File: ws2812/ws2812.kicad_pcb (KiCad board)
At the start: 2 copper layers, 76.2 x 50.8 mm, 8 parts, among them J1 STM32WORLD_BASE, J2 STM32WORLD_CONNECTOR_1, J3 STM32WORLD_CONNECTOR_2, U1 WS2812E, U2 WS2812E, U3 WS2812E, U4 WS2812E, U5 WS2812E

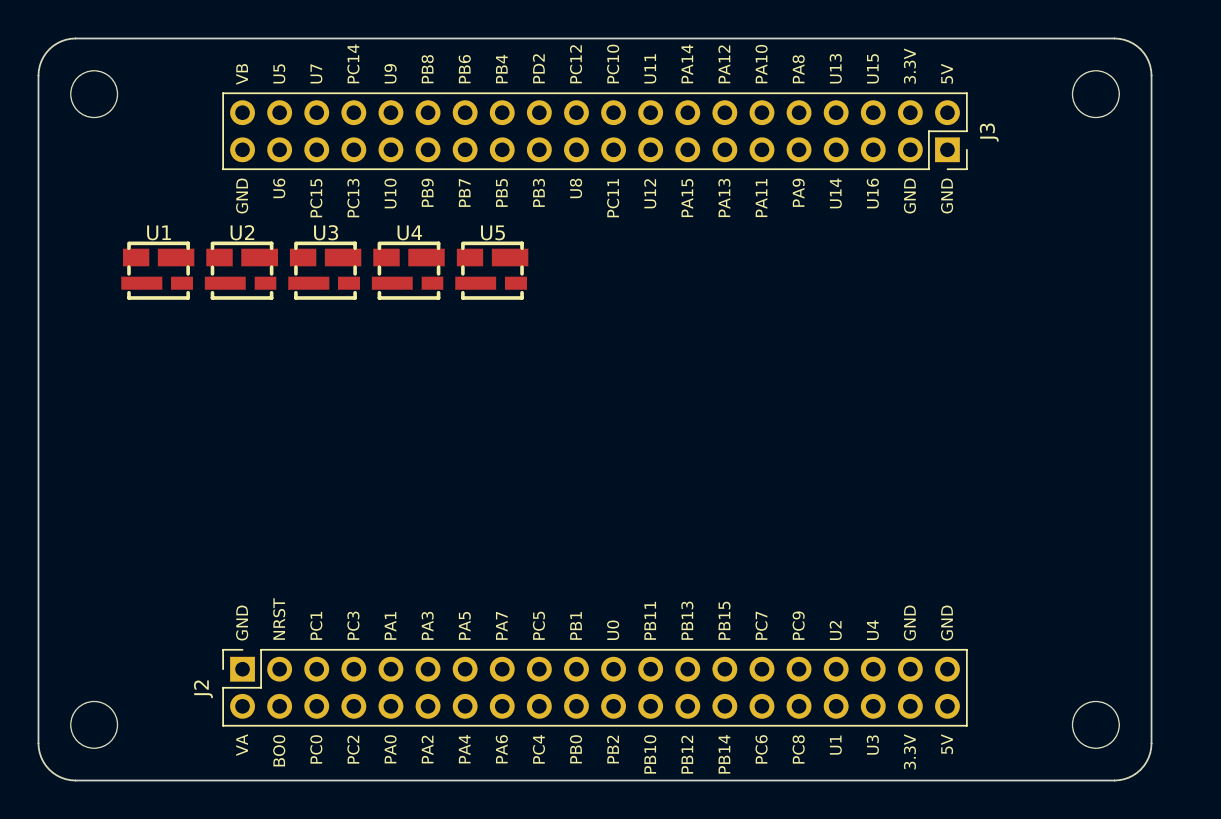
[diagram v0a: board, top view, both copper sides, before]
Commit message: Hmmmm
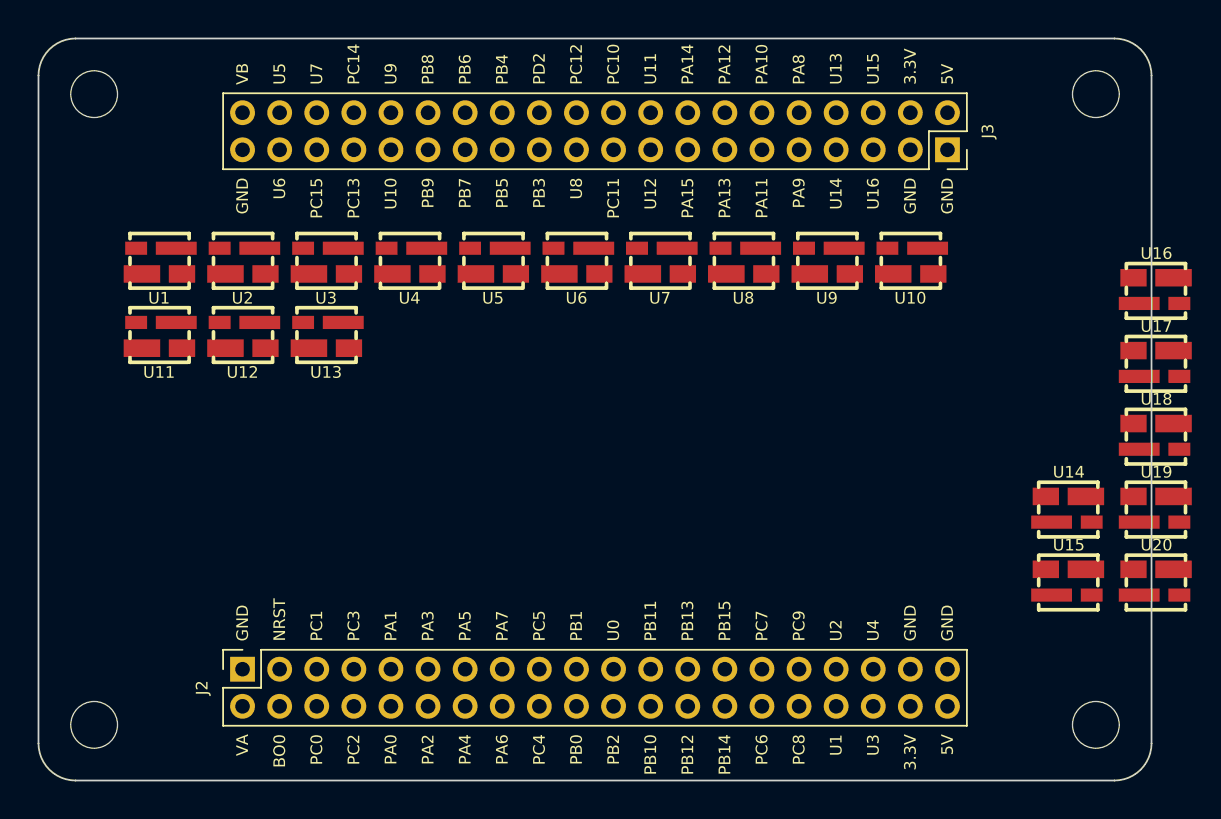
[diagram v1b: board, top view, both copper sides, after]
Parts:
- added U10: WS2812E, stm32world:LED-SMD_4P-L3.7-W3.5-P1.75-BR-SK6812MINI, F.Cu at (167.6, 85.1)
- added U11: WS2812E, stm32world:LED-SMD_4P-L3.7-W3.5-P1.75-BR-SK6812MINI, F.Cu at (116.2, 90.2)
- added U12: WS2812E, stm32world:LED-SMD_4P-L3.7-W3.5-P1.75-BR-SK6812MINI, F.Cu at (121.9, 90.2)
- added U13: WS2812E, stm32world:LED-SMD_4P-L3.7-W3.5-P1.75-BR-SK6812MINI, F.Cu at (127.6, 90.2)
- added U14: WS2812E, stm32world:LED-SMD_4P-L3.7-W3.5-P1.75-BR-SK6812MINI, F.Cu at (178.5, 102.1)
- added U15: WS2812E, stm32world:LED-SMD_4P-L3.7-W3.5-P1.75-BR-SK6812MINI, F.Cu at (178.5, 107.1)
- added U16: WS2812E, stm32world:LED-SMD_4P-L3.7-W3.5-P1.75-BR-SK6812MINI, F.Cu at (184.5, 87.1)
- added U17: WS2812E, stm32world:LED-SMD_4P-L3.7-W3.5-P1.75-BR-SK6812MINI, F.Cu at (184.5, 92.1)
- added U18: WS2812E, stm32world:LED-SMD_4P-L3.7-W3.5-P1.75-BR-SK6812MINI, F.Cu at (184.5, 97.1)
- added U19: WS2812E, stm32world:LED-SMD_4P-L3.7-W3.5-P1.75-BR-SK6812MINI, F.Cu at (184.5, 102.1)
- added U20: WS2812E, stm32world:LED-SMD_4P-L3.7-W3.5-P1.75-BR-SK6812MINI, F.Cu at (184.5, 107.1)
- added U6: WS2812E, stm32world:LED-SMD_4P-L3.7-W3.5-P1.75-BR-SK6812MINI, F.Cu at (144.8, 85.1)
- added U7: WS2812E, stm32world:LED-SMD_4P-L3.7-W3.5-P1.75-BR-SK6812MINI, F.Cu at (150.5, 85.1)
- added U8: WS2812E, stm32world:LED-SMD_4P-L3.7-W3.5-P1.75-BR-SK6812MINI, F.Cu at (156.2, 85.1)
- added U9: WS2812E, stm32world:LED-SMD_4P-L3.7-W3.5-P1.75-BR-SK6812MINI, F.Cu at (161.9, 85.1)
- J1: value STM32WORLD_BASE -> STM32WORLD_BOARD
- moved U1 0.63 mm to (116.2, 85.1), turned to 180 degrees
- moved U2 0.63 mm to (121.9, 85.1), turned to 180 degrees
- moved U3 0.63 mm to (127.6, 85.1), turned to 180 degrees
- moved U4 0.63 mm to (133.3, 85.1), turned to 180 degrees
- moved U5 0.63 mm to (139.1, 85.1), turned to 180 degrees
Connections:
- U1 pad 2: unconnected-(U1-VDD-Pad2) -> VCC
- U1 pad 3: unconnected-(U1-DO-Pad3) -> Net-(U1-DO)
- U1 pad 4: unconnected-(U1-GND-Pad4) -> GND
- U2 pad 1: unconnected-(U2-DI-Pad1) -> Net-(U1-DO)
- U2 pad 2: unconnected-(U2-VDD-Pad2) -> VCC
- U2 pad 3: unconnected-(U2-DO-Pad3) -> Net-(U2-DO)
- U2 pad 4: unconnected-(U2-GND-Pad4) -> GND
- U3 pad 1: unconnected-(U3-DI-Pad1) -> Net-(U2-DO)
- U3 pad 2: unconnected-(U3-VDD-Pad2) -> VCC
- U3 pad 3: unconnected-(U3-DO-Pad3) -> Net-(U3-DO)
- U3 pad 4: unconnected-(U3-GND-Pad4) -> GND
- U4 pad 1: unconnected-(U4-DI-Pad1) -> Net-(U3-DO)
- U4 pad 2: unconnected-(U4-VDD-Pad2) -> VCC
- U4 pad 3: unconnected-(U4-DO-Pad3) -> Net-(U4-DO)
- U4 pad 4: unconnected-(U4-GND-Pad4) -> GND
- U5 pad 1: unconnected-(U5-DI-Pad1) -> Net-(U4-DO)
- U5 pad 2: unconnected-(U5-VDD-Pad2) -> VCC
- U5 pad 3: unconnected-(U5-DO-Pad3) -> Net-(U5-DO)
- U5 pad 4: unconnected-(U5-GND-Pad4) -> GND

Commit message: More
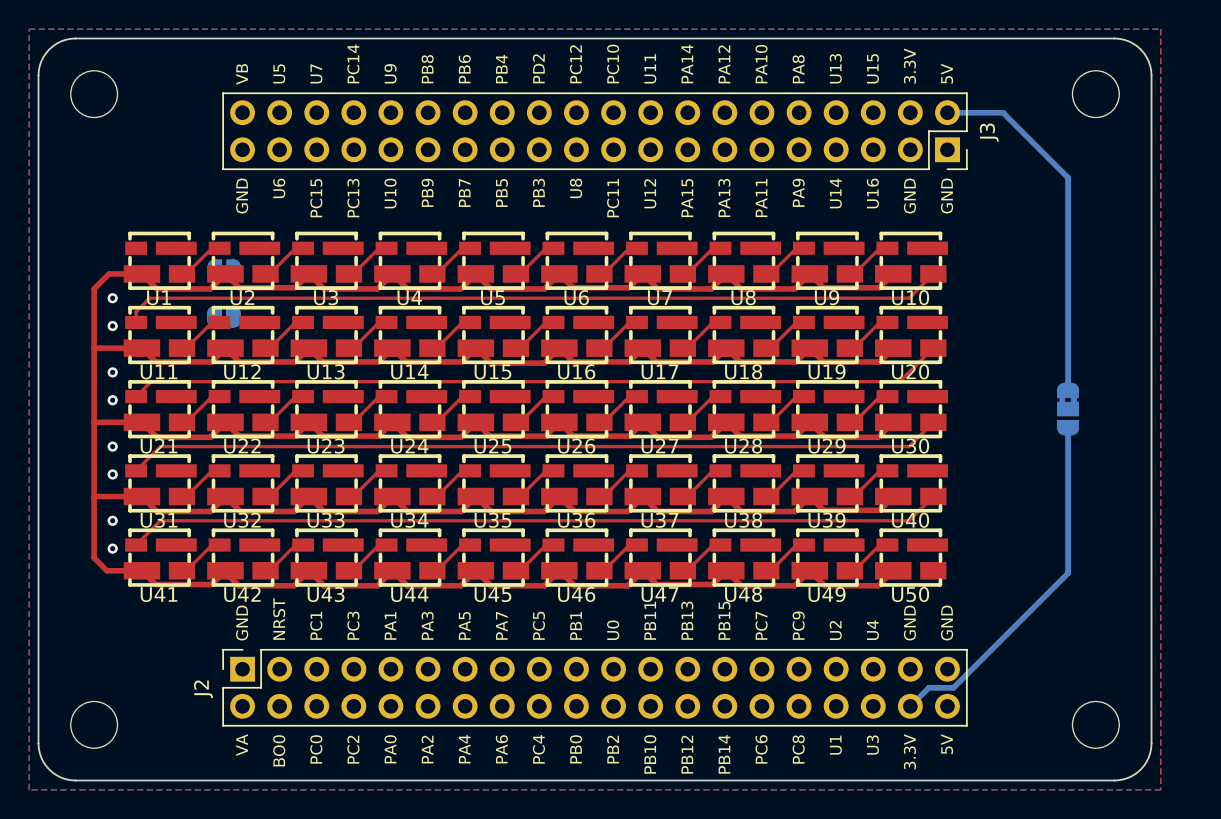
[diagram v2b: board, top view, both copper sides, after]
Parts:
- added JP1: ~, Jumper:SolderJumper-3_P1.3mm_Bridged2Bar12_RoundedPad1.0x1.5mm, B.Cu at (178.4, 95.2)
- added JP2: ~, Jumper:SolderJumper-2_P1.3mm_Open_RoundedPad1.0x1.5mm, B.Cu at (120.7, 85.7)
- added JP3: ~, Jumper:SolderJumper-2_P1.3mm_Open_RoundedPad1.0x1.5mm, B.Cu at (120.7, 88.9)
- added U21: WS2812E, stm32world:LED-SMD_4P-L3.7-W3.5-P1.75-BR-SK6812MINI, F.Cu at (116.2, 95.2)
- added U22: WS2812E, stm32world:LED-SMD_4P-L3.7-W3.5-P1.75-BR-SK6812MINI, F.Cu at (121.9, 95.2)
- added U23: WS2812E, stm32world:LED-SMD_4P-L3.7-W3.5-P1.75-BR-SK6812MINI, F.Cu at (127.6, 95.2)
- added U24: WS2812E, stm32world:LED-SMD_4P-L3.7-W3.5-P1.75-BR-SK6812MINI, F.Cu at (133.3, 95.2)
- added U25: WS2812E, stm32world:LED-SMD_4P-L3.7-W3.5-P1.75-BR-SK6812MINI, F.Cu at (139.1, 95.2)
- added U26: WS2812E, stm32world:LED-SMD_4P-L3.7-W3.5-P1.75-BR-SK6812MINI, F.Cu at (144.8, 95.2)
- added U27: WS2812E, stm32world:LED-SMD_4P-L3.7-W3.5-P1.75-BR-SK6812MINI, F.Cu at (150.5, 95.2)
- added U28: WS2812E, stm32world:LED-SMD_4P-L3.7-W3.5-P1.75-BR-SK6812MINI, F.Cu at (156.2, 95.2)
- added U29: WS2812E, stm32world:LED-SMD_4P-L3.7-W3.5-P1.75-BR-SK6812MINI, F.Cu at (161.9, 95.2)
- added U30: WS2812E, stm32world:LED-SMD_4P-L3.7-W3.5-P1.75-BR-SK6812MINI, F.Cu at (167.6, 95.2)
- added U31: WS2812E, stm32world:LED-SMD_4P-L3.7-W3.5-P1.75-BR-SK6812MINI, F.Cu at (116.2, 100.3)
- added U32: WS2812E, stm32world:LED-SMD_4P-L3.7-W3.5-P1.75-BR-SK6812MINI, F.Cu at (121.9, 100.3)
- added U33: WS2812E, stm32world:LED-SMD_4P-L3.7-W3.5-P1.75-BR-SK6812MINI, F.Cu at (127.6, 100.3)
- added U34: WS2812E, stm32world:LED-SMD_4P-L3.7-W3.5-P1.75-BR-SK6812MINI, F.Cu at (133.3, 100.3)
- added U35: WS2812E, stm32world:LED-SMD_4P-L3.7-W3.5-P1.75-BR-SK6812MINI, F.Cu at (139.1, 100.3)
- added U36: WS2812E, stm32world:LED-SMD_4P-L3.7-W3.5-P1.75-BR-SK6812MINI, F.Cu at (144.8, 100.3)
- added U37: WS2812E, stm32world:LED-SMD_4P-L3.7-W3.5-P1.75-BR-SK6812MINI, F.Cu at (150.5, 100.3)
- added U38: WS2812E, stm32world:LED-SMD_4P-L3.7-W3.5-P1.75-BR-SK6812MINI, F.Cu at (156.2, 100.3)
- added U39: WS2812E, stm32world:LED-SMD_4P-L3.7-W3.5-P1.75-BR-SK6812MINI, F.Cu at (161.9, 100.3)
- added U40: WS2812E, stm32world:LED-SMD_4P-L3.7-W3.5-P1.75-BR-SK6812MINI, F.Cu at (167.6, 100.3)
- added U41: WS2812E, stm32world:LED-SMD_4P-L3.7-W3.5-P1.75-BR-SK6812MINI, F.Cu at (116.2, 105.4)
- added U42: WS2812E, stm32world:LED-SMD_4P-L3.7-W3.5-P1.75-BR-SK6812MINI, F.Cu at (121.9, 105.4)
- added U43: WS2812E, stm32world:LED-SMD_4P-L3.7-W3.5-P1.75-BR-SK6812MINI, F.Cu at (127.6, 105.4)
- added U44: WS2812E, stm32world:LED-SMD_4P-L3.7-W3.5-P1.75-BR-SK6812MINI, F.Cu at (133.3, 105.4)
- added U45: WS2812E, stm32world:LED-SMD_4P-L3.7-W3.5-P1.75-BR-SK6812MINI, F.Cu at (139.1, 105.4)
- added U46: WS2812E, stm32world:LED-SMD_4P-L3.7-W3.5-P1.75-BR-SK6812MINI, F.Cu at (144.8, 105.4)
- added U47: WS2812E, stm32world:LED-SMD_4P-L3.7-W3.5-P1.75-BR-SK6812MINI, F.Cu at (150.5, 105.4)
- added U48: WS2812E, stm32world:LED-SMD_4P-L3.7-W3.5-P1.75-BR-SK6812MINI, F.Cu at (156.2, 105.4)
- added U49: WS2812E, stm32world:LED-SMD_4P-L3.7-W3.5-P1.75-BR-SK6812MINI, F.Cu at (161.9, 105.4)
- added U50: WS2812E, stm32world:LED-SMD_4P-L3.7-W3.5-P1.75-BR-SK6812MINI, F.Cu at (167.6, 105.4)
- moved U14 46.7 mm to (133.3, 90.2), turned to 180 degrees
- moved U15 42.9 mm to (139.1, 90.2), turned to 180 degrees
- moved U16 39.8 mm to (144.8, 90.2), turned to 180 degrees
- moved U17 34.0 mm to (150.5, 90.2), turned to 180 degrees
- moved U18 29.1 mm to (156.2, 90.2), turned to 180 degrees
- moved U19 25.5 mm to (161.9, 90.2), turned to 180 degrees
- moved U20 23.9 mm to (167.6, 90.2), turned to 180 degrees
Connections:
- J2 pad 1: unconnected-(J2-GND-Pad1) -> GND
- J2 pad 10: unconnected-(J2-PA0-Pad10) -> TIM5_1
- J2 pad 37: unconnected-(J2-GND-Pad37) -> GND
- J2 pad 38: unconnected-(J2-3.3V-Pad38) -> +3.3V
- J2 pad 39: unconnected-(J2-GND-Pad39) -> GND
- J2 pad 40: unconnected-(J2-5V-Pad40) -> +5V
- J2 pad 9: unconnected-(J2-PA1-Pad9) -> TIM5_2
- J3 pad 1: unconnected-(J3-GND-Pad1) -> GND
- J3 pad 2: unconnected-(J3-5V-Pad2) -> +5V
- J3 pad 3: unconnected-(J3-GND-Pad3) -> GND
- J3 pad 4: unconnected-(J3-3.3V-Pad4) -> +3.3V
- U1 pad 1: unconnected-(U1-DI-Pad1) -> LED
- U10 pad 3: unconnected-(U10-DO-Pad3) -> Net-(U10-DO)
- U11 pad 1: unconnected-(U11-DI-Pad1) -> Net-(U10-DO)
- U20 pad 3: unconnected-(U20-DO-Pad3) -> Net-(U20-DO)
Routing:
- net VCC: track 0.00 -> 329.8 mm
- net Net-(U10-DO): track 0.00 -> 56.4 mm
- net Net-(U40-DO): track 0.00 -> 56.0 mm
- net Net-(U30-DO): track 0.00 -> 56.0 mm
- net Net-(U20-DO): track 0.00 -> 56.0 mm
- net +5V: track 0.00 -> 24.6 mm
- net +3.3V: track 0.00 -> 24.5 mm
- net Net-(U6-DO): track 0.00 -> 3.30 mm
- net Net-(U5-DO): track 0.00 -> 3.30 mm
- net Net-(U46-DO): track 0.00 -> 3.30 mm
- net Net-(U45-DO): track 0.00 -> 3.30 mm
- net Net-(U44-DO): track 0.00 -> 3.30 mm
- net Net-(U4-DO): track 0.00 -> 3.30 mm
- net Net-(U36-DO): track 0.00 -> 3.30 mm
- net Net-(U35-DO): track 0.00 -> 3.30 mm
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- added copper zone on B.Cu, net GND
- added copper zone on F.Cu, net GND
